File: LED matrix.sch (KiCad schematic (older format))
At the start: 61 parts

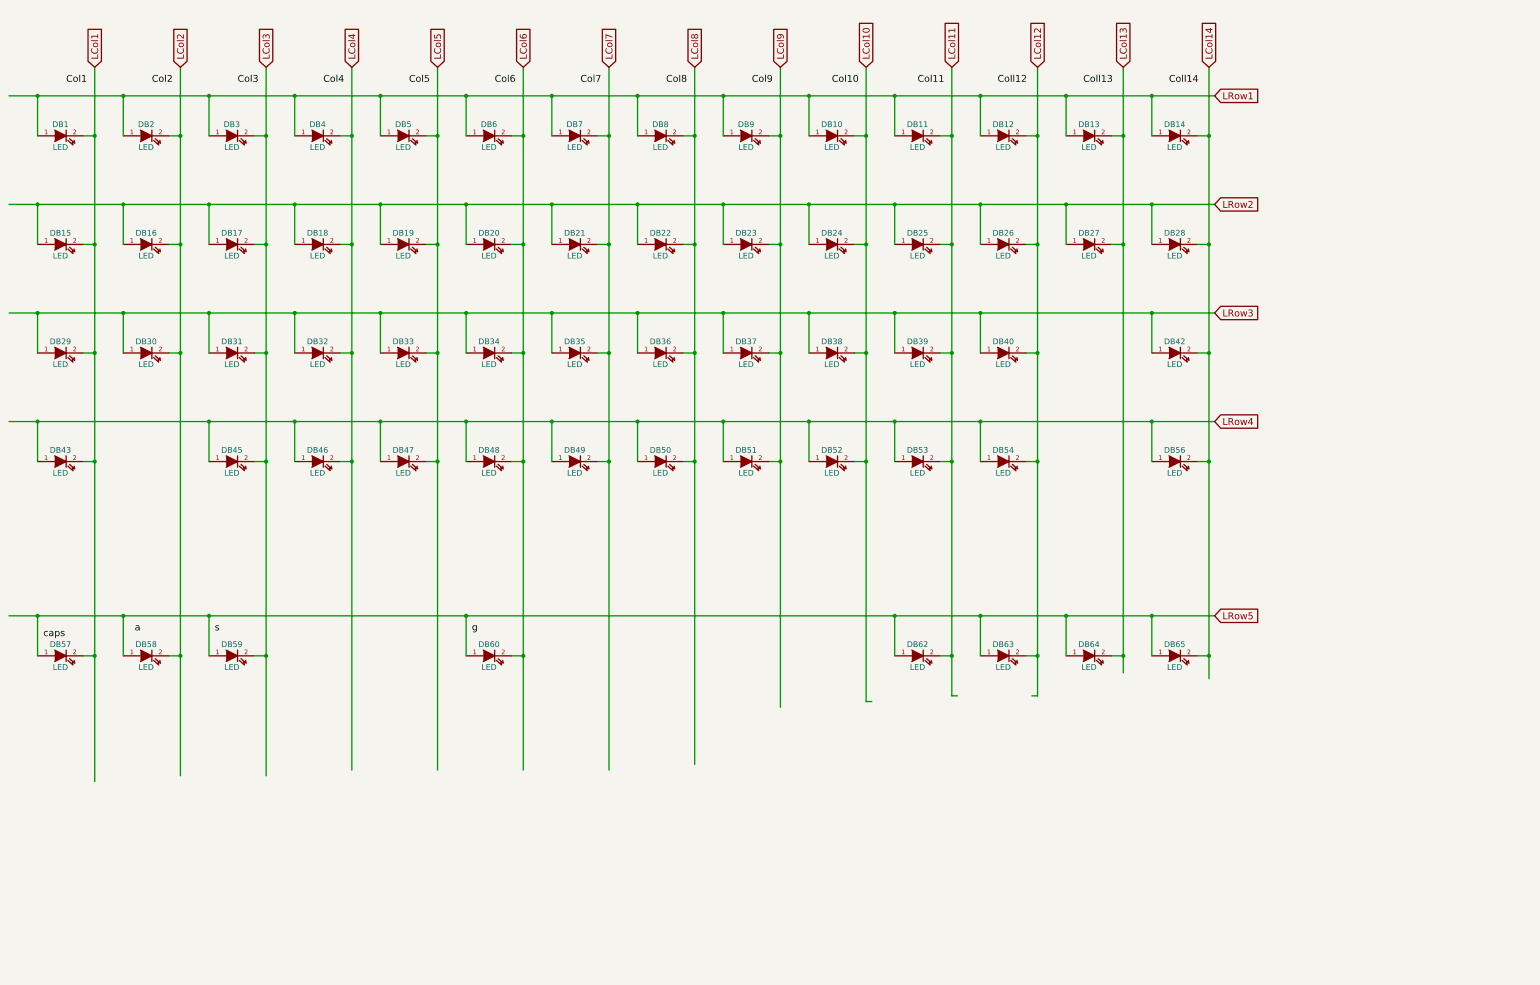
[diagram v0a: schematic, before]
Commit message: Add files via upload
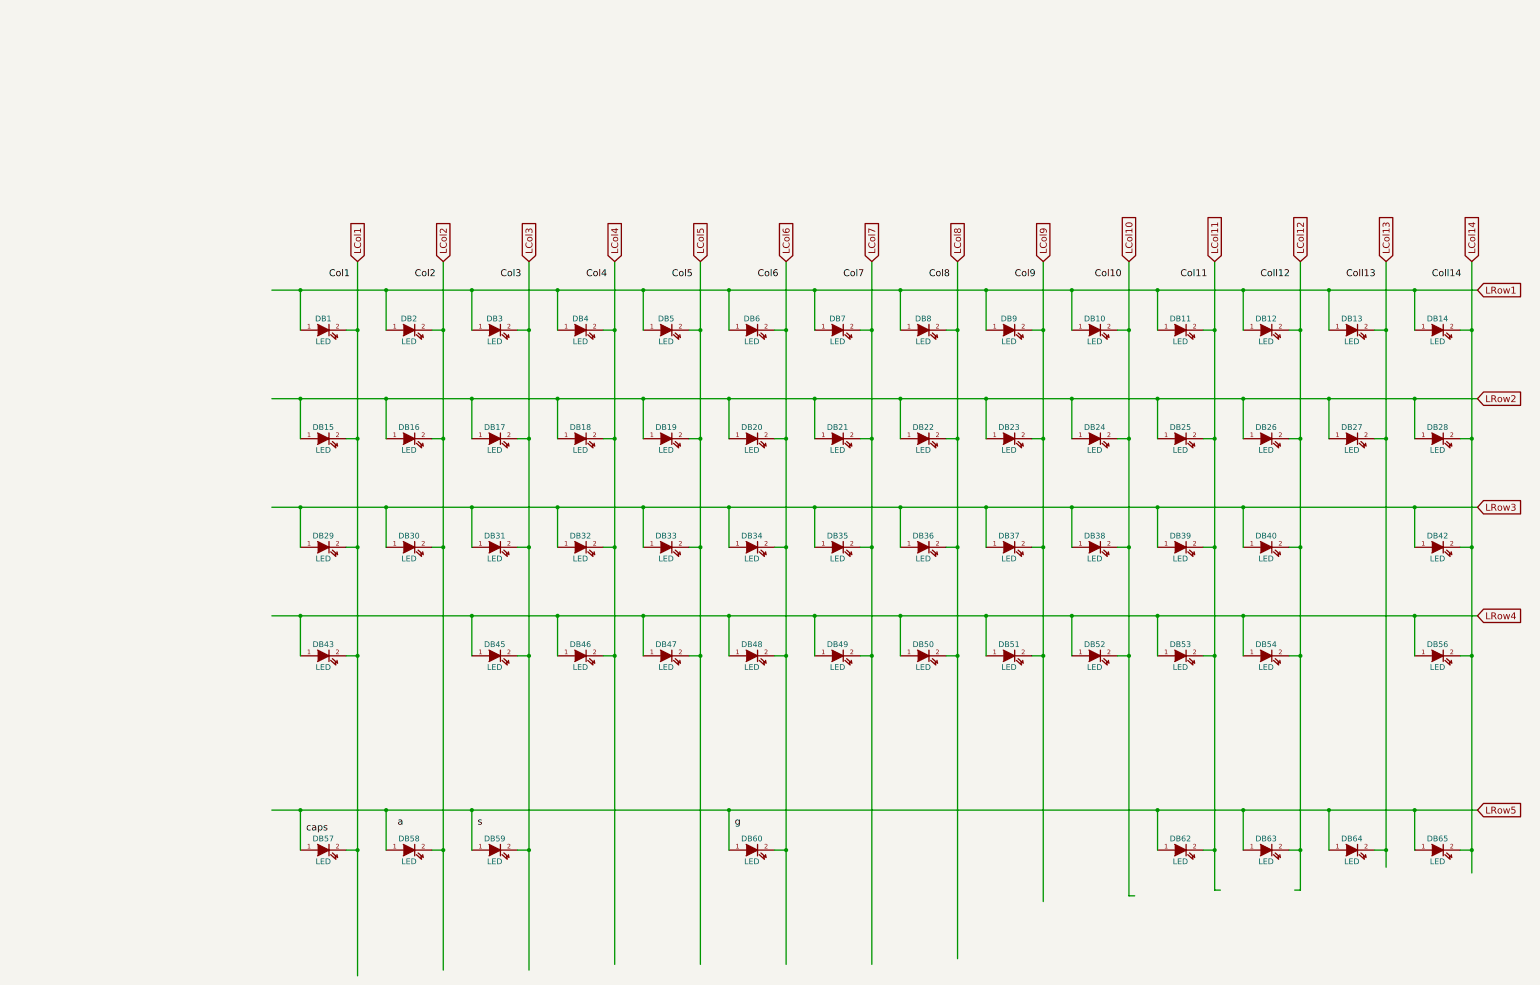
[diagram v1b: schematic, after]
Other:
- moved on the sheet: DB1, DB10, DB11, DB12, DB13, DB14, DB15, DB16, DB17, DB18, DB19, DB2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
